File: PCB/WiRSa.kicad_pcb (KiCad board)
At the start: 2 copper layers, 51.3 x 31.5 mm, 14 parts, among them SW1 SW_Push, SW2 SW_Push, SW3 SW_Push, SW4 SW_Push, U1 WeMos_D1_mini

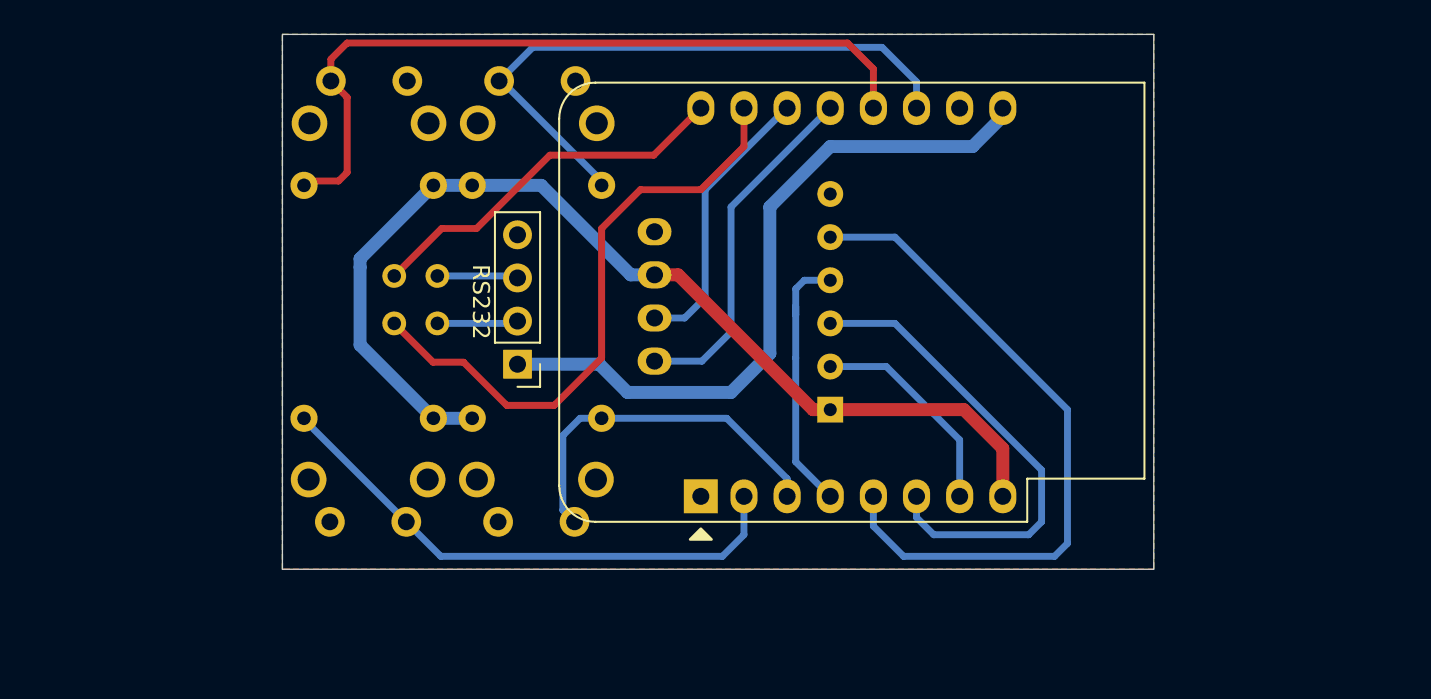
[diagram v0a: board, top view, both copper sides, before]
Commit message: WiRSa v3.01
Initial push for the version 3 design
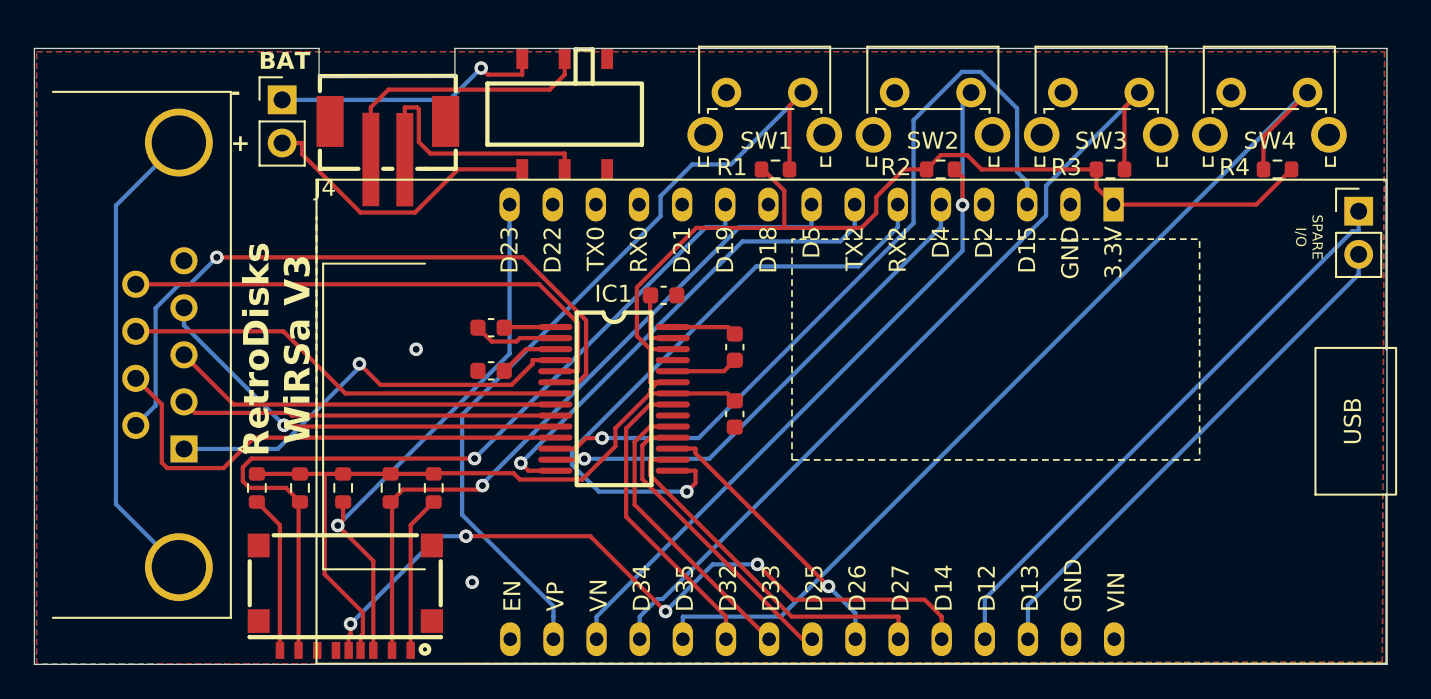
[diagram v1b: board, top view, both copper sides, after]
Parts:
- removed A1: SD_Card_Module, Charles:SD_Card_Module
- removed Brd1: SSD1306, SSD1306:128x64OLED
- removed RS232: RS232_TTL_Adapter, Connector_PinHeader_2.54mm:PinHeader_1x04_P2.54mm_Vertical
- removed RX: RX, TestPoint:TestPoint_2Pads_Pitch2.54mm_Drill0.8mm
- removed TX: TX, TestPoint:TestPoint_2Pads_Pitch2.54mm_Drill0.8mm
- added C1: 0.1uF, Capacitor_SMD:C_0603_1608Metric, F.Cu at (87.1, 91.1)
- added C2: 0.1uF, Capacitor_SMD:C_0603_1608Metric, F.Cu at (72.7, 89.9)
- added C3: 0.1uF, Capacitor_SMD:C_0603_1608Metric, F.Cu at (82.9, 88.0)
- added C4: 0.1uF, Capacitor_SMD:C_0603_1608Metric, F.Cu at (87.1, 95.0)
- added C5: 0.1uF, Capacitor_SMD:C_0603_1608Metric, F.Cu at (72.7, 92.5)
- added G***: LOGO, wirsa:retrodisks, B.Cu at (63.4, 92.6)
- added IC1: MAX3243CDBR, easyeda2kicad:SSOP-28_L10.2-W5.3-P0.65-LS7.8-BL, F.Cu at (80.0, 94.1)
- added J1: DE9 Female, Connector_Dsub:DSUB-9_Female_Horizontal_P2.77x2.84mm_EdgePinOffset4.94mm_Housed_MountingHolesOffset7.48mm, F.Cu at (54.7, 97.1)
- added J2: spare IO, Connector_PinHeader_2.54mm:PinHeader_1x02_P2.54mm_Vertical, F.Cu at (123.8, 83.1)
- added J3: Conn_01x02_Socket, Connector_PinHeader_2.54mm:PinHeader_1x02_P2.54mm_Vertical, F.Cu at (60.4, 76.5)
- added J4: 2016WVS-02P, easyeda2kicad:CONN-SMD_P2.00_X2016WVS-02-9TSW, F.Cu at (66.7, 78.9)
- added R5: 10k, Resistor_SMD:R_0603_1608Metric, F.Cu at (58.9, 99.4)
- added R6: 10k, Resistor_SMD:R_0603_1608Metric, F.Cu at (61.5, 99.4)
- added R7: 10k, Resistor_SMD:R_0603_1608Metric, F.Cu at (64.0, 99.4)
- added R8: 10k, Resistor_SMD:R_0603_1608Metric, F.Cu at (66.8, 99.4)
- added R9: 10k, Resistor_SMD:R_0603_1608Metric, F.Cu at (69.4, 99.4)
- added SW5: SK-3245S-L3-B, easyeda2kicad:SW-SMD_SK-3245S-L3-B, F.Cu at (77.1, 77.3)
- added U2: ESP32-WROOM-32D DEV BOARD, esp32:ESP32-C3-DevKitC-02, F.Cu at (62.5, 109.7)
- R1, R2, R3, R4: footprint Resistor_THT:R_Axial_DIN0207_L6.3mm_D2.5mm_P7.62mm_Horizontal -> Resistor_SMD:R_0603_1608Metric; moved to F.Cu
- SW1, SW2, SW3, SW4: moved to F.Cu
- U1: value WeMos_D1_mini -> TF-123-ARP9H17; footprint Module:WEMOS_D1_mini_light -> easyeda2kicad:TF-SMD_TF-123-ARP9H15
- moved R4 47.4 mm to (119.0, 80.6), turned to 180 degrees
- moved R3 39.9 mm to (109.2, 80.6), turned to 0 degrees
- moved SW4 38.6 mm to (116.3, 76.1), turned to 0 degrees
- moved SW3 38.6 mm to (106.4, 76.1), turned to 0 degrees
- moved SW2 34.4 mm to (96.5, 76.1)
- moved SW1 34.4 mm to (86.6, 76.1)
- moved R2 31.2 mm to (99.2, 80.6)
- moved R1 24.9 mm to (89.5, 80.6), turned to 0 degrees
- moved U1 21.8 mm to (64.2, 105.8), turned to 0 degrees
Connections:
- R1 pad 1: Net-(A1-Pad1) -> Net-(IC1-FORCEON)
- R1 pad 2: Net-(R1-Pad2) -> Net-(U2-D36/SENS_VP)
- R2 pad 1: Net-(A1-Pad1) -> Net-(IC1-FORCEON)
- R2 pad 2: Net-(R2-Pad2) -> Net-(U2-D39/SENS_VN)
- R3 pad 1: Net-(A1-Pad1) -> Net-(IC1-FORCEON)
- R3 pad 2: Net-(R3-Pad2) -> Net-(U2-D34)
- R4 pad 1: Net-(A1-Pad1) -> Net-(IC1-FORCEON)
- R4 pad 2: Net-(R4-Pad2) -> Net-(U2-D35)
- SW1 pad 2: Net-(R1-Pad2) -> Net-(U2-D36/SENS_VP)
- SW2 pad 2: Net-(R2-Pad2) -> Net-(U2-D39/SENS_VN)
- SW3 pad 2: Net-(R3-Pad2) -> Net-(U2-D34)
- SW4 pad 2: Net-(R4-Pad2) -> Net-(U2-D35)
- U1 pad 1: unconnected-(U1-Pad1) -> Net-(U1-DAT2)
- U1 pad 11: Net-(R4-Pad2) -> GND
- U1 pad 12: Net-(R3-Pad2) -> GND
- U1 pad 13: Net-(Brd1-Pad4) -> GND
- U1 pad 2: Net-(R1-Pad2) -> Net-(U1-CD/DAT3)
- U1 pad 3: Net-(R2-Pad2) -> Net-(U1-CMD)
- U1 pad 4: Net-(A1-Pad4) -> Net-(IC1-FORCEON)
- U1 pad 6: Net-(A1-Pad3) -> GND
- U1 pad 8: Net-(A1-Pad1) -> Net-(U1-DAT1)
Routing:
- net Net-(IC1-FORCEON): track 0.00 -> 101.3 mm
- net Net-(A1-Pad1): track 62.3 -> 0.00 mm
- net Net-(U2-D35): track 0.00 -> 56.5 mm
- net Net-(U2-D34): track 0.00 -> 49.4 mm
- net Net-(U2-D36/SENS_VP): track 0.00 -> 48.9 mm
- net /RTS-TI: track 0.00 -> 46.7 mm, vias 0 -> 1
- net Net-(R3-Pad2): track 45.1 -> 0.00 mm
- net Net-(U2-D39/SENS_VN): track 0.00 -> 43.6 mm, vias 0 -> 1
- net Net-(U1-CD/DAT3): track 0.00 -> 41.6 mm, vias 0 -> 1
- net /DSR-RI: track 0.00 -> 40.7 mm, vias 0 -> 1
- net Net-(U1-CLK): track 40.3 -> 0.00 mm
- net /RX-TO: track 0.00 -> 37.0 mm, vias 0 -> 1
- net Net-(U1-DAT0): track 12.7 -> 49.1 mm, vias 0 -> 1
- net Net-(R4-Pad2): track 36.3 -> 0.00 mm
- net Net-(JP1-Pad2): track 35.6 -> 0.00 mm
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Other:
- board size 51.3 x 31.5 mm -> 79.6 x 36.3 mm
- board text added: "+"
- board text added: "-"
- board text added: "BAT"
- board text added: "CTS (RI)"
- board text added: "DCD (RI)"
- board text added: "DSR (RI)"
- board text added: "DTR (RO)"
- board text added: "GND"
- board text added: "RI (RI)"
- board text added: "RTS (RO)"
- board text added: "RX (RI)"
- board text added: "RetroDisks WiRSa V3"
- board text added: "SPARE I/O"
- board text added: "TX (RO)"
- board text added: "WiRSa V3"
- board text removed: "RetroDisks WiRSa v2"
